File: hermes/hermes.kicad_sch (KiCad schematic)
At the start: 8 parts, among them U1 AHT20, U2 XIAO-RP2040-DIP

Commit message: changed some footprints
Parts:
- C1: footprint Capacitor_SMD:C_0402_1005Metric -> Capacitor_THT:CP_Radial_D5.0mm_P2.00mm
- R1, R2, R3: footprint Resistor_SMD:R_0402_1005Metric -> Resistor_THT:R_Axial_DIN0207_L6.3mm_D2.5mm_P10.16mm_Horizontal
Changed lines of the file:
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@@
 			)
 		)
-		(property "Footprint" "Resistor_SMD:R_0402_1005Metric"
+		(property "Footprint" "Resistor_THT:R_Axial_DIN0207_L6.3mm_D2.5mm_P10.16mm_Horizontal"
 			(at 155.702 93.98 90)
 			(effects
@@
 			)
 		)
-		(property "Footprint" "Resistor_SMD:R_0402_1005Metric"
+		(property "Footprint" "Resistor_THT:R_Axial_DIN0207_L6.3mm_D2.5mm_P10.16mm_Horizontal"
 			(at 206.502 92.71 90)
 			(effects
@@
 			)
 		)
-		(property "Footprint" "Resistor_SMD:R_0402_1005Metric"
+		(property "Footprint" "Resistor_THT:R_Axial_DIN0207_L6.3mm_D2.5mm_P10.16mm_Horizontal"
 			(at 160.782 93.98 90)
 			(effects
@@
 			)
 		)
-		(property "Footprint" "Capacitor_SMD:C_0402_1005Metric"
+		(property "Footprint" "Capacitor_THT:CP_Radial_D5.0mm_P2.00mm"
 			(at 209.2452 107.95 0)
 			(effects

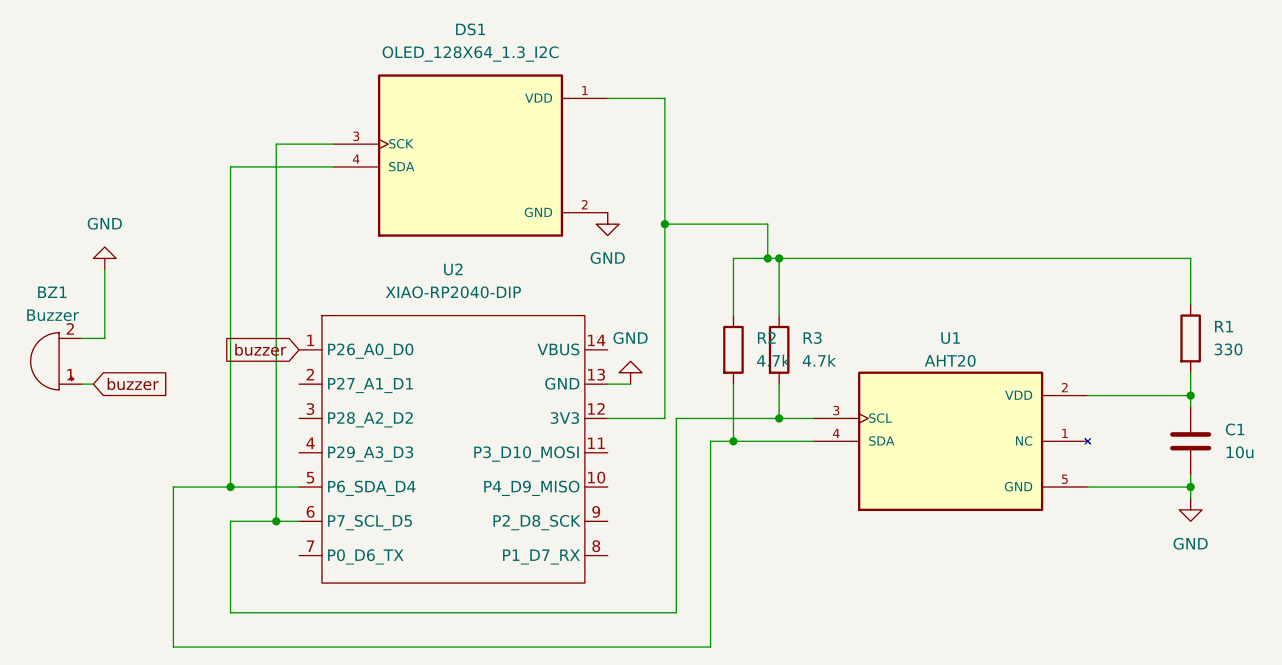
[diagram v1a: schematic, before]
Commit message: done
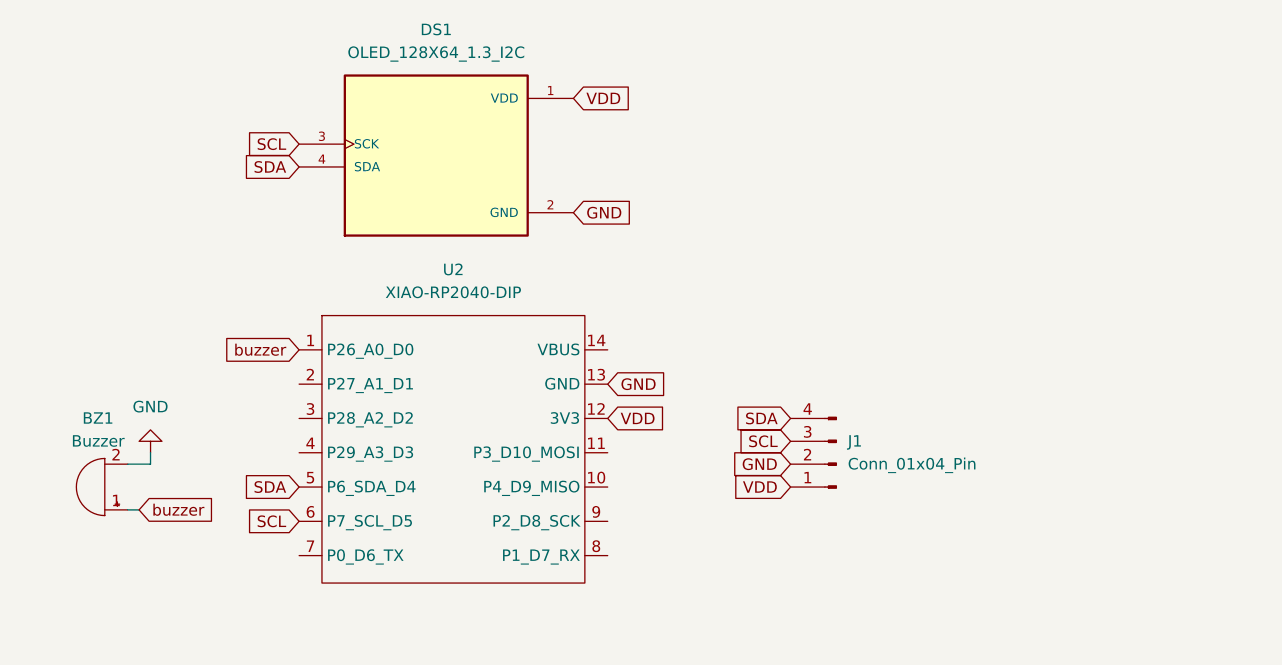
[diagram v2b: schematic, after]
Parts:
- removed C1: 10u, Capacitor_THT:CP_Radial_D5.0mm_P2.00mm, symbol Device:C
- removed R1: 330, Resistor_THT:R_Axial_DIN0207_L6.3mm_D2.5mm_P10.16mm_Horizontal, symbol Device:R
- removed R2, R3: 4.7k, Resistor_THT:R_Axial_DIN0207_L6.3mm_D2.5mm_P10.16mm_Horizontal, symbol Device:R
- removed U1: AHT20, hermes-footprint:PSON100P300X300X110-6N, symbol AHT20:AHT20
- added J1: Conn_01x04_Pin, Connector:FanPinHeader_1x04_P2.54mm_Vertical, symbol Connector:Conn_01x04_Pin
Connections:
- net GND: now also J1.2 (Pin_2)
- net VDD: now reaches DS1.1 (VDD), U2.12 (3V3)
- net VDD: now also J1.1 (Pin_1)
- net SDA: now reaches DS1.4 (SDA), U2.5 (P6_SDA_D4)
- net SDA: now also J1.4 (Pin_4)
- net SCL: now reaches DS1.3 (SCK), U2.6 (P7_SCL_D5)
- net SCL: now also J1.3 (Pin_3)
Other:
- moved on the sheet: BZ1, DS1

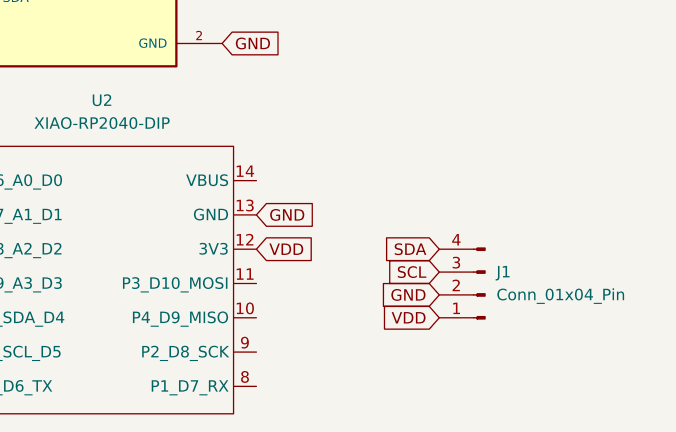
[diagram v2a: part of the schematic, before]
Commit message: made a case
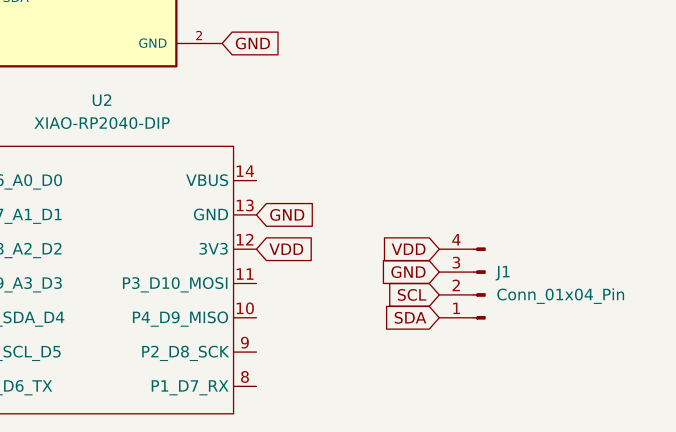
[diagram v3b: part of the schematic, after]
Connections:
- net GND: now also J1.3 (Pin_3); no longer J1.2 (Pin_2)
- net SCL: now also J1.2 (Pin_2); no longer J1.3 (Pin_3)
- net SDA: now also J1.1 (Pin_1); no longer J1.4 (Pin_4)
- net VDD: now also J1.4 (Pin_4); no longer J1.1 (Pin_1)
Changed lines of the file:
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@@
 		)
 	)
-	(global_label "GND"
+	(global_label "SCL"
 		(shape input)
 		(at 163.83 106.68 180)
@@
 		)
 		(property "Intersheetrefs" "${INTERSHEET_REFS}"
-			(at 156.9743 106.68 0)
+			(at 157.3372 106.68 0)
 			(effects
 				(font
@@
 		)
 	)
-	(global_label "VDD"
+	(global_label "SDA"
 		(shape input)
 		(at 163.83 109.22 180)
@@
 		)
 		(property "Intersheetrefs" "${INTERSHEET_REFS}"
-			(at 157.2162 109.22 0)
+			(at 157.2767 109.22 0)
 			(effects
 				(font
@@
 		)
 	)
-	(global_label "SCL"
+	(global_label "GND"
 		(shape input)
 		(at 163.83 104.14 180)
@@
 		)
 		(property "Intersheetrefs" "${INTERSHEET_REFS}"
-			(at 157.3372 104.14 0)
+			(at 156.9743 104.14 0)
 			(effects
 				(font
@@
 		)
 	)
-	(global_label "SDA"
+	(global_label "VDD"
 		(shape input)
 		(at 163.83 101.6 180)
@@
 		)
 		(property "Intersheetrefs" "${INTERSHEET_REFS}"
-			(at 157.2767 101.6 0)
+			(at 157.2162 101.6 0)
 			(effects
 				(font
